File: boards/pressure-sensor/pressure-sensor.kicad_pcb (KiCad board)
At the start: 2 copper layers, 25.9 x 23.4 mm, 5 parts, among them J1 CONN_01X04_MALE, M3 MountingHole_3.2mm_M3

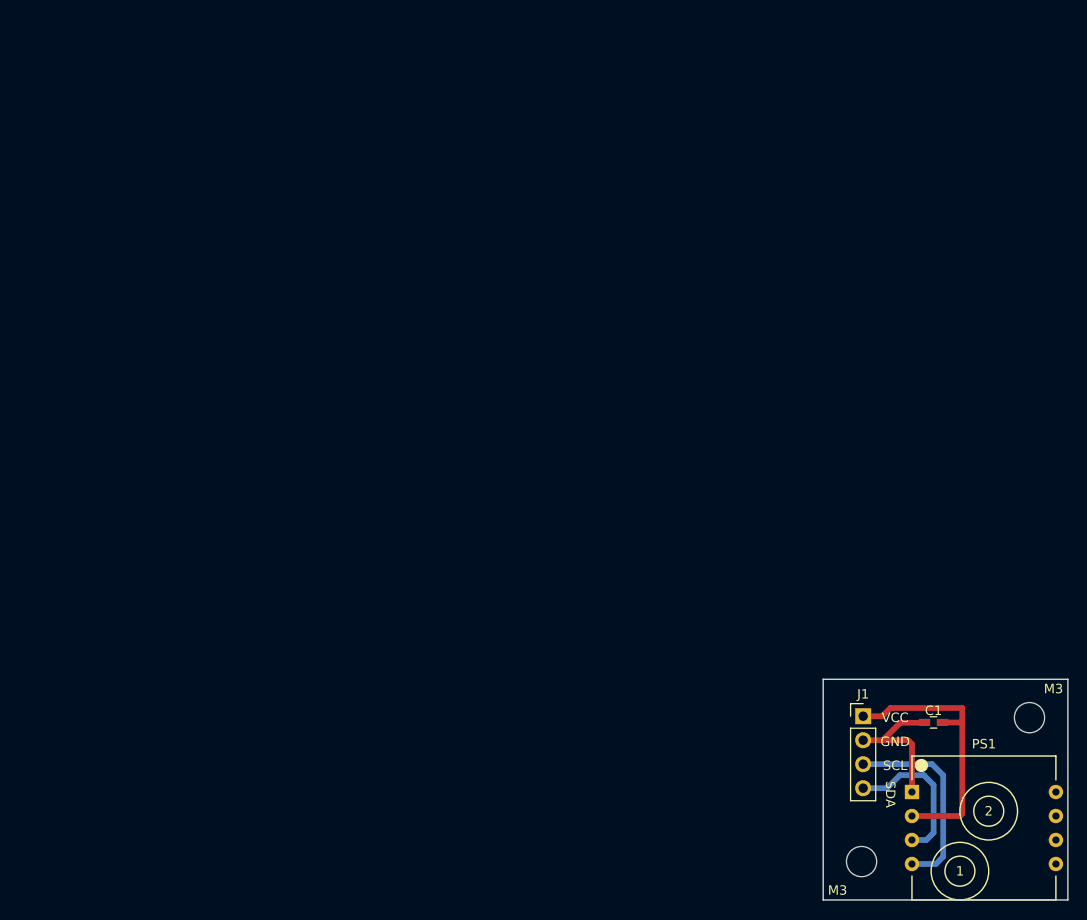
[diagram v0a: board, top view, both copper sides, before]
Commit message: [docs] export all board layouts
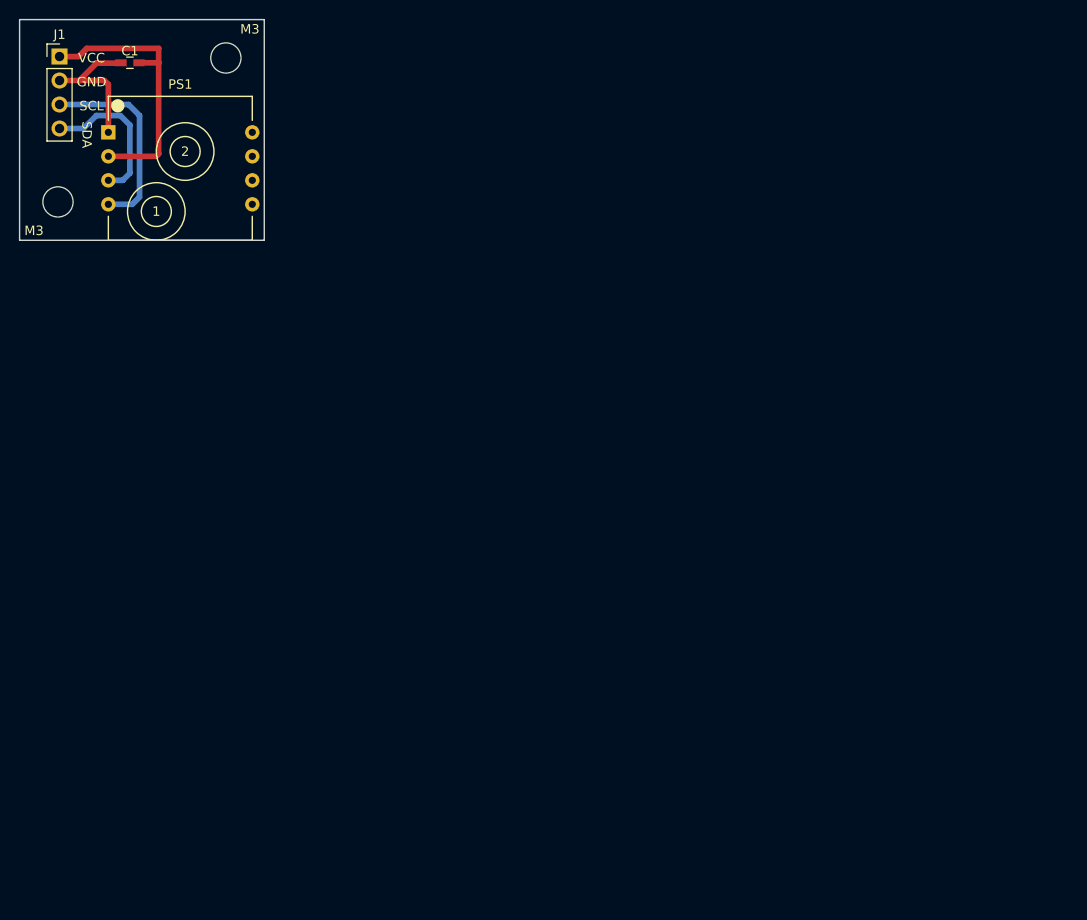
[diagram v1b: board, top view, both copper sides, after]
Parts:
- moved J1 110.1 mm to (63.4, 35.2)
- moved M3 110.1 mm to (81.0, 35.3)
- moved C1 110.1 mm to (70.9, 35.8)
- moved M3 110.1 mm to (63.2, 50.5)
- moved PS1 110.1 mm to (68.6, 39.4)
